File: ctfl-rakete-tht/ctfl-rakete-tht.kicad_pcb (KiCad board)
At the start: 2 copper layers, 99.8 x 99.4 mm, 21 parts, among them J1 Conn_02x03_Odd_Even, SW1 SW_SPDT, U1 ATtiny212-SS

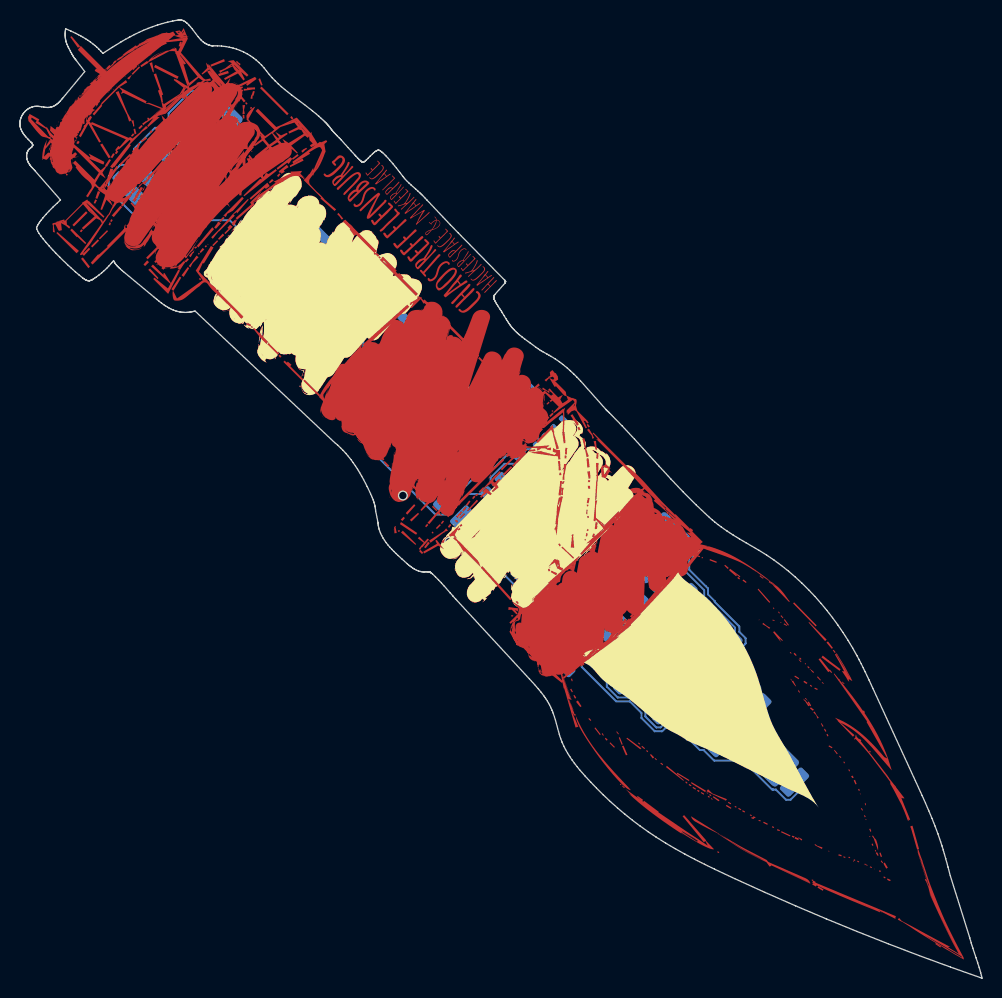
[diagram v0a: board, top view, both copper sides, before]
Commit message: finished layout for revision A
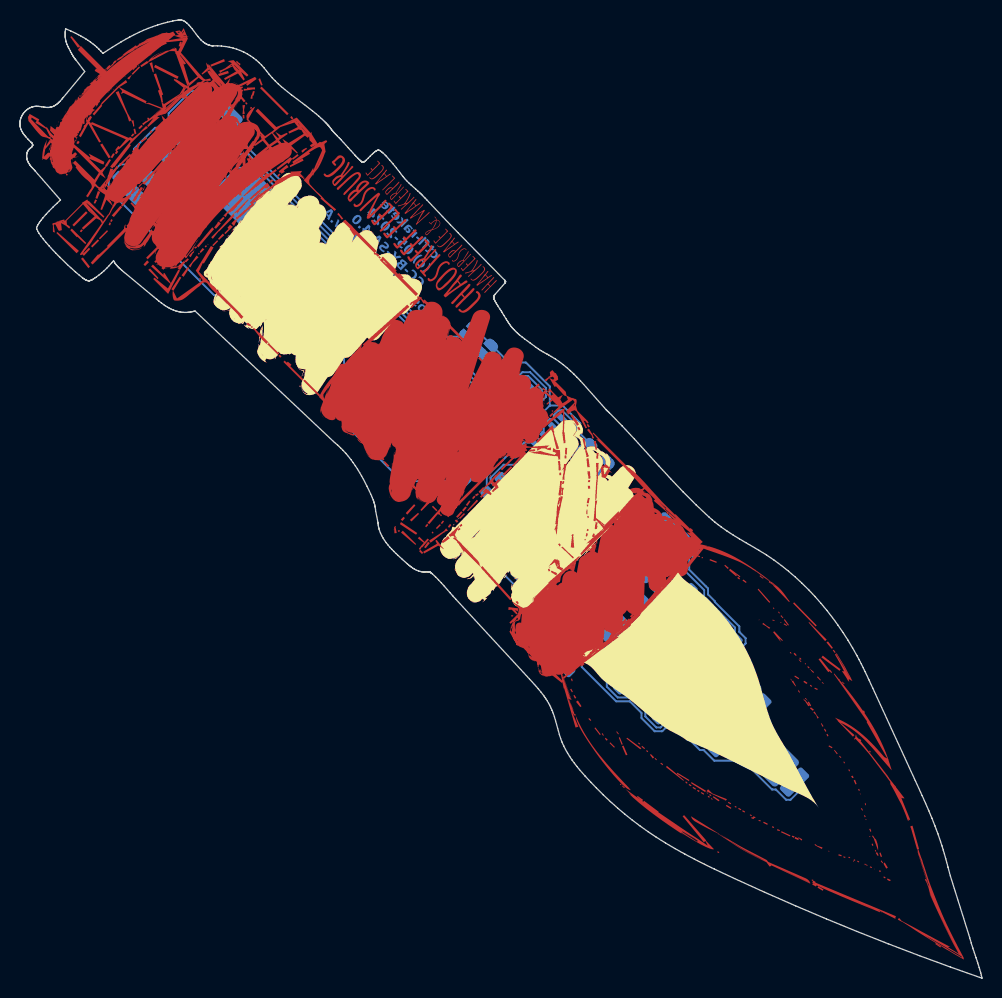
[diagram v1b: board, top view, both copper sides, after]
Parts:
- added JP1: SolderJumper_2_Open, Jumper:SolderJumper-2_P1.3mm_Open_RoundedPad1.0x1.5mm, B.Cu at (146.5, 93.5)
- added JP2: SolderJumper_2_Open, Jumper:SolderJumper-2_P1.3mm_Open_RoundedPad1.0x1.5mm, B.Cu at (150.3, 86.2)
- added JP3: SolderJumper_2_Open, Jumper:SolderJumper-2_P1.3mm_Open_RoundedPad1.0x1.5mm, B.Cu at (148.5, 84.4)
- added JP4: SolderJumper_2_Open, Jumper:SolderJumper-2_P1.3mm_Open_RoundedPad1.0x1.5mm, B.Cu at (146.7, 82.6)
- added JP5: SolderJumper_2_Open, Jumper:SolderJumper-2_P1.3mm_Open_RoundedPad1.0x1.5mm, B.Cu at (158.8, 94.7)
- added JP6: SolderJumper_2_Open, Jumper:SolderJumper-2_P1.3mm_Open_RoundedPad1.0x1.5mm, B.Cu at (160.6, 96.5)
- SW1: footprint Button_Switch_SMD:SW_SPDT_CK_JS102011SAQN -> local:SW_SPDT_ESP4020
- moved SW1 3.31 mm to (142.0, 98.6)
- moved BT1 2.83 mm to (133.7, 78.7)
- moved C1 0.28 mm to (150.8, 94.1)
- moved U1 0.28 mm to (153.5, 91.4)
- moved D1 0.05 mm to (111.2, 65.9)
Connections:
- U1 pad 2: /flame_inner -> /light_left
- U1 pad 3: /flame_outer -> /light_center
- U1 pad 4: /light_left -> /light_right
- U1 pad 5: /light_center -> /flame_outer
- U1 pad 7: /light_right -> /flame_inner
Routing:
- net /light_left: track 3.04 -> 65.0 mm
- net /light_center: track 3.04 -> 62.4 mm
- net /light_right: track 3.04 -> 49.3 mm
- net /flame_inner: track 43.9 -> 72.5 mm
- net +3V0: track 33.9 -> 58.5 mm
- net /flame_outer: track 74.0 -> 92.1 mm
- net GND: track 210.4 -> 211.8 mm
- net Net-(BT1-+): track 37.5 -> 38.4 mm
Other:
- board text added: "100n"
- board text added: "4k7"
- board text added: "ATTINY212"
- board text added: "CR2023"
- board text added: "GND"
- board text added: "LEDs on"
- board text added: "OFF"
- board text added: "ON"
- board text added: "PWR"
- board text added: "UPDI"
- board text added: "VCC"
- board text added: "ctfl-rakete (c) 05-2024 CC-BY-SA 4.0 Jost Salathé - Rev.A"
